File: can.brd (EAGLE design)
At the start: 65.7 x 29.2 mm, 32 parts, among them J1 AVR_SPI_PRG_6NS, Q1 FDS5680, Q2 FDS5680, Q3 FDS5680, U1 ATMEGA8, U2 MCP2510SO, U3 MCP2551SN

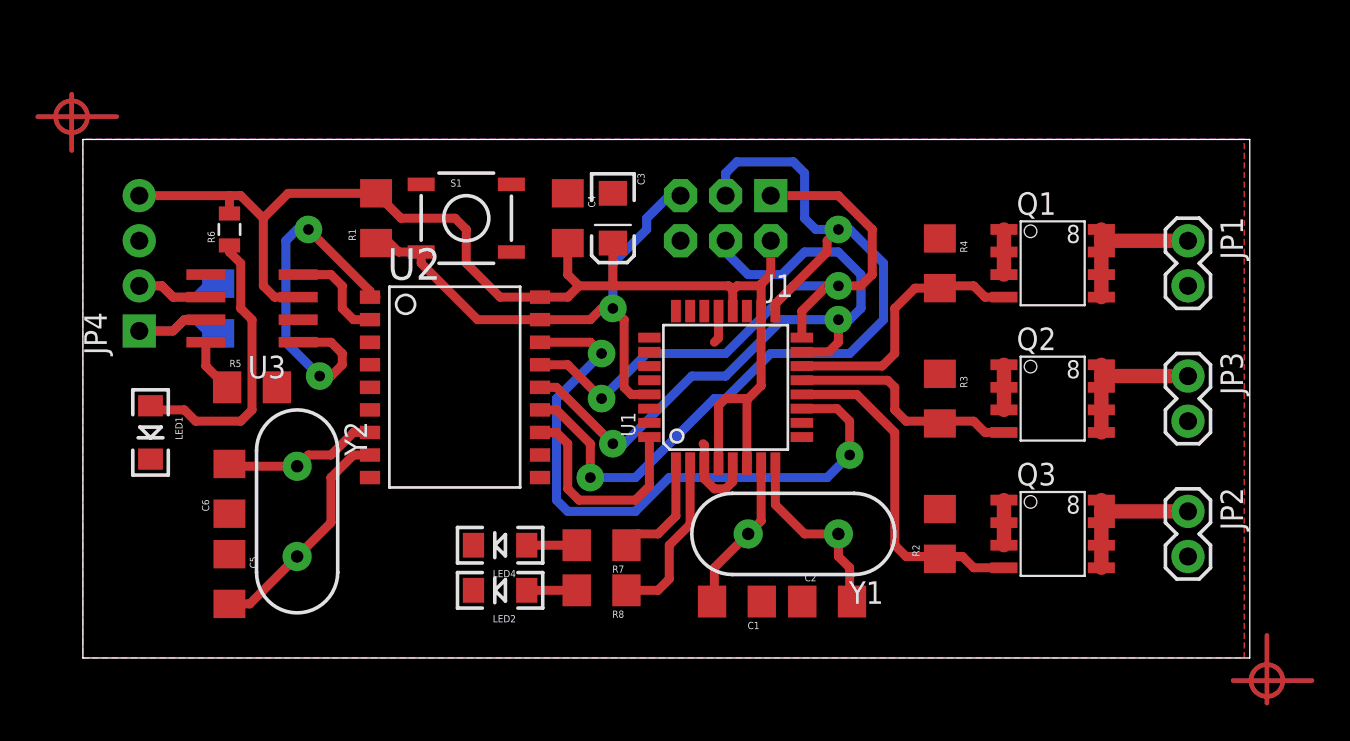
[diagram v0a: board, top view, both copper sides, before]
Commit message: 1.0.0
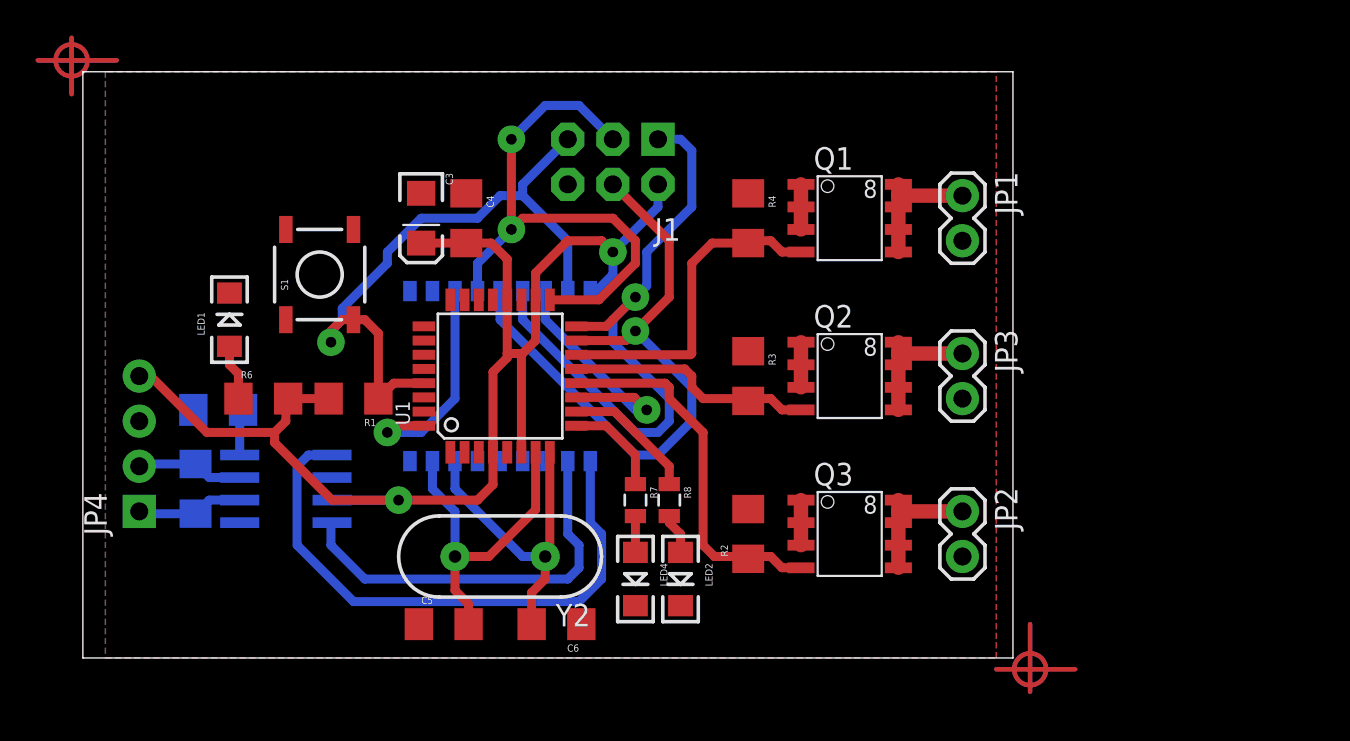
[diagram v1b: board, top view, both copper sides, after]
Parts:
- removed C1, C2: (no value), SparkFun-Capacitors:1206
- removed Y1: (no value), SparkFun-FreqCtrl:HC49US
- R6: device SparkFun-Passives:0805 -> SparkFun-Passives:1206
- R7, R8: device SparkFun-Resistors:1206 -> SparkFun-Resistors:0805
- moved C6 19.9 mm to (26.7, 1.91), turned to 180 degrees
- moved JP1 13.0 mm to (49.5, 26.0)
- moved JP3 12.8 mm to (49.5, 17.1)
- moved U1 12.7 mm to (23.5, 15.9)
- moved JP2 12.7 mm to (49.5, 8.26)
- moved C5 12.3 mm to (20.3, 1.91), turned to 0 degrees
- moved Y2 11.7 mm to (23.5, 5.71), turned to 180 degrees
- moved Q1 11.7 mm to (43.2, 24.8)
- moved Q2 11.5 mm to (43.2, 15.9)
- moved Q3 11.4 mm to (43.2, 6.99)
- moved R4 11.1 mm to (37.5, 24.8)
- moved R3 10.9 mm to (37.5, 15.9)
- moved C3 10.8 mm to (19.1, 24.8)
- moved R2 10.8 mm to (37.5, 6.99)
- moved U3 10.3 mm to (11.4, 9.53), flipped to the bottom, turned to 270 degrees
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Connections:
- removed net N$12: R8.1, U1.2
- removed net N$4: C1.2, U1.7, Y1.2
- removed net N$5: C2.2, U1.8, Y1.1
- removed net N$9: R7.1, U1.1
- new net OSC1: C5.2, U1.7, U2.8, Y2.2
- new net OSC2: C6.2, U1.8, U2.7, Y2.1
- net CANH: now also JP4.2; no longer JP4.1
- net CANL: now also JP4.1; no longer JP4.2
- net N$1: now also R8.1, U1.10; no longer C5.2, U2.8, Y2.2
- net N$3: now also R7.1, U1.9; no longer C6.2, U2.7, Y2.1
- net RS: now also R5.2; no longer R5.1
- net VSS: now also R5.1; no longer C1.1, C2.1, R5.2
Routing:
- net SS: track 36.0 -> 13.7 mm, vias 2 -> 1
- net OSC1: track 0.00 -> 18.9 mm
- net OSC2: track 0.00 -> 18.3 mm
- net SCK: track 49.2 -> 31.3 mm
- net RXCAN: track 5.84 -> 22.6 mm
- net N$13: track 16.1 -> 3.15 mm
- net TXCAN: track 20.4 -> 32.6 mm, vias 2 -> 0
- net N$5: track 10.7 -> 0.00 mm
- net N$12: track 9.66 -> 0.00 mm
- net N$4: track 8.92 -> 0.00 mm
- net VSS: track 14.5 -> 7.62 mm
- net N$9: track 6.42 -> 0.00 mm
- net RESET: track 31.0 -> 36.5 mm
- net N$1: track 12.9 -> 7.51 mm
- net N$7: track 15.0 -> 18.5 mm
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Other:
- board size 65.7 x 29.2 mm -> 52.4 x 33 mm
